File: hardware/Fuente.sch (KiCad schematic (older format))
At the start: 3 parts

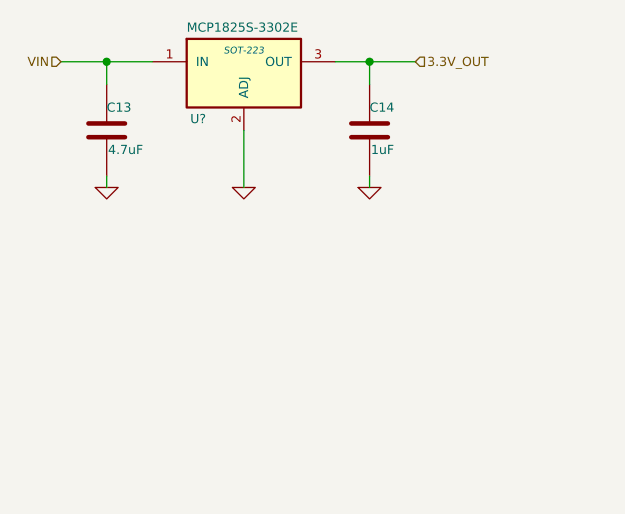
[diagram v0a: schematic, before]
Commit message: Terminado el esquematico, iniciado el PCB
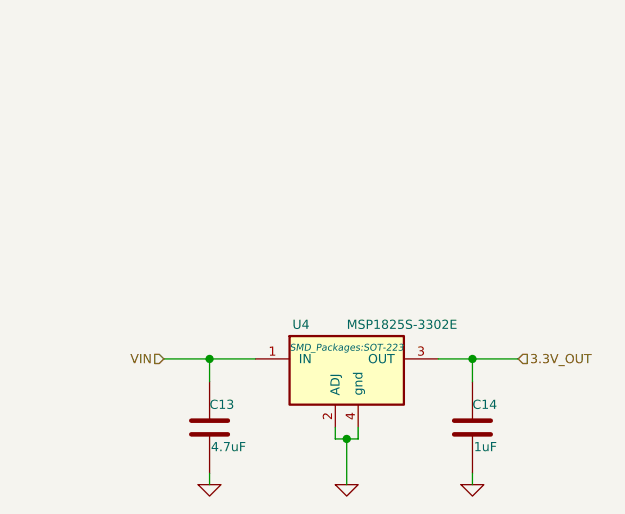
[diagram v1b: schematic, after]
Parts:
- removed U?: MCP1825S-3302E, SOT-223, symbol LM117H
- added U4: MSP1825S-3302E, SMD_Packages:SOT-223, symbol MSP1825S-3302E
- C13, C14: footprint (none) -> Capacitors_ThroughHole:Capacitor5x11RM2.5
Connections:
- net 3.3V_OUT: now also U4.3 (OUT)
- net GND: now also U4.2 (ADJ), U4.4 (gnd)
- net VIN: now also U4.1 (IN)
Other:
- moved on the sheet: C13, C14
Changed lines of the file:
@@
 L C C14
 U 1 1 53D55294
-P 5900 2550
-F 0 "C14" H 5900 2650 40  0000 L CNN
-F 1 "1uF" H 5906 2465 40  0000 L CNN
-F 2 "" H 5938 2400 30  0000 C CNN
-F 3 "" H 5900 2550 60  0000 C CNN
-	1    5900 2550
+P 6350 3850
+F 0 "C14" H 6350 3950 40  0000 L CNN
+F 1 "1uF" H 6356 3765 40  0000 L CNN
+F 2 "Capacitors_ThroughHole:Capacitor5x11RM2.5" H 6388 3700 30  0001 C CNN
+F 3 "" H 6350 3850 60  0000 C CNN
+	1    6350 3850
 	1    0    0    -1
 $EndComp
@@
 L C C13
 U 1 1 53D552E9
-P 4750 2550
-F 0 "C13" H 4750 2650 40  0000 L CNN
-F 1 "4.7uF" H 4756 2465 40  0000 L CNN
-F 2 "" H 4788 2400 30  0000 C CNN
-F 3 "" H 4750 2550 60  0000 C CNN
-	1    4750 2550
+P 5200 3850
+F 0 "C13" H 5200 3950 40  0000 L CNN
+F 1 "4.7uF" H 5206 3765 40  0000 L CNN
+F 2 "Capacitors_ThroughHole:Capacitor5x11RM2.5" H 5238 3700 30  0001 C CNN
+F 3 "" H 5200 3850 60  0000 C CNN
+	1    5200 3850
 	1    0    0    -1
 $EndComp
 Wire Wire Line
-	4550 2250 4750 2250
+	5000 3550 5400 3550
 Wire Wire Line
-	4750 2250 4950 2250
+	6200 3550 6550 3550
 Wire Wire Line
-	5750 2250 5900 2250
-Wire Wire Line
-	5900 2250 6100 2250
-Wire Wire Line
-	4750 2350 4750 2250
-Connection ~ 4750 2250
+	5200 3650 5200 3550
+Connection ~ 5200 3550
 $Comp
-L GND #PWR52
+L GND #PWR051
 U 1 1 53D555A6
-P 4750 2800
-F 0 "#PWR52" H 4750 2800 30  0001 C CNN
-F 1 "GND" H 4750 2730 30  0001 C CNN
-F 2 "" H 4750 2800 60  0000 C CNN
-F 3 "" H 4750 2800 60  0000 C CNN
-	1    4750 2800
+P 5200 4100
+F 0 "#PWR051" H 5200 4100 30  0001 C CNN
+F 1 "GND" H 5200 4030 30  0001 C CNN
+F 2 "" H 5200 4100 60  0000 C CNN
+F 3 "" H 5200 4100 60  0000 C CNN
+	1    5200 4100
 	1    0    0    -1
 $EndComp
 Wire Wire Line
-	4750 2800 4750 2750
+	5200 4100 5200 4050
 $Comp
-L GND #PWR55
+L GND #PWR052
 U 1 1 53D555D6
-P 5900 2800
-F 0 "#PWR55" H 5900 2800 30  0001 C CNN
-F 1 "GND" H 5900 2730 30  0001 C CNN
-F 2 "" H 5900 2800 60  0000 C CNN
-F 3 "" H 5900 2800 60  0000 C CNN
-	1    5900 2800
+P 6350 4100
+F 0 "#PWR052" H 6350 4100 30  0001 C CNN
+F 1 "GND" H 6350 4030 30  0001 C CNN
+F 2 "" H 6350 4100 60  0000 C CNN
+F 3 "" H 6350 4100 60  0000 C CNN
+	1    6350 4100
 	1    0    0    -1
 $EndComp
 Wire Wire Line
-	5900 2800 5900 2750
+	6350 4100 6350 4050
 $Comp
-L GND #PWR53
+L GND #PWR053
 U 1 1 53D55626
-P 5350 2800
-F 0 "#PWR53" H 5350 2800 30  0001 C CNN
-F 1 "GND" H 5350 2730 30  0001 C CNN
-F 2 "" H 5350 2800 60  0000 C CNN
-F 3 "" H 5350 2800 60  0000 C CNN
-	1    5350 2800
+P 5800 4100
+F 0 "#PWR053" H 5800 4100 30  0001 C CNN
+F 1 "GND" H 5800 4030 30  0001 C CNN
+F 2 "" H 5800 4100 60  0000 C CNN
+F 3 "" H 5800 4100 60  0000 C CNN
+	1    5800 4100
 	1    0    0    -1
 $EndComp
+Connection ~ 6350 3550
+Text HLabel 6550 3550 2    40   Input ~ 0
+3.3V_OUT
 Wire Wire Line
-	5350 2800 5350 2550
-Connection ~ 5900 2250
+	6350 3650 6350 3550
+Text HLabel 5000 3550 0    40   Input ~ 0
+VIN
+Wire Wire Line
+	5850 3850 5850 3900
+Wire Wire Line
+	5850 3900 5750 3900
+Wire Wire Line
+	5750 3900 5750 3850
+Wire Wire Line
+	5800 3900 5800 4100
+Connection ~ 5800 3900
 $Comp
-L LM117H U?
-U 1 1 53DE486A
-P 5350 2300
-F 0 "U?" H 5150 2100 40  0000 C CNN
-F 1 "MCP1825S-3302E" H 5100 2500 40  0000 L CNN
-F 2 "SOT-223" H 5350 2400 30  0000 C CIN
-F 3 "" H 5350 2300 60  0000 C CNN
-	1    5350 2300
+L MSP1825S-3302E U4
+U 1 1 53E687BD
+P 5800 3600
+F 0 "U4" H 5600 3800 40  0000 C CNN
+F 1 "MSP1825S-3302E" H 5800 3800 40  0000 L CNN
+F 2 "SMD_Packages:SOT-223" H 5800 3700 30  0000 C CIN
+F 3 "" H 5800 3600 60  0000 C CNN
+	1    5800 3600
 	1    0    0    -1
 $EndComp
-Text HLabel 6100 2250 2    40   Input ~ 0
-3.3V_OUT
-Wire Wire Line
-	5900 2350 5900 2250
-Text HLabel 4550 2250 0    40   Input ~ 0
-VIN
 $EndSCHEMATC
